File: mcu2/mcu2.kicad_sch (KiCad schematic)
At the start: 35 parts, among them J1 KF128-5.08, J2 Conn_01x30, J8 Conn_01x30, Q1 WSF3085, Q2 PL4009, Q3 PL4009, U1 Pico, U2 motor_driver, U3 max31865_module, U4 dcdc_module

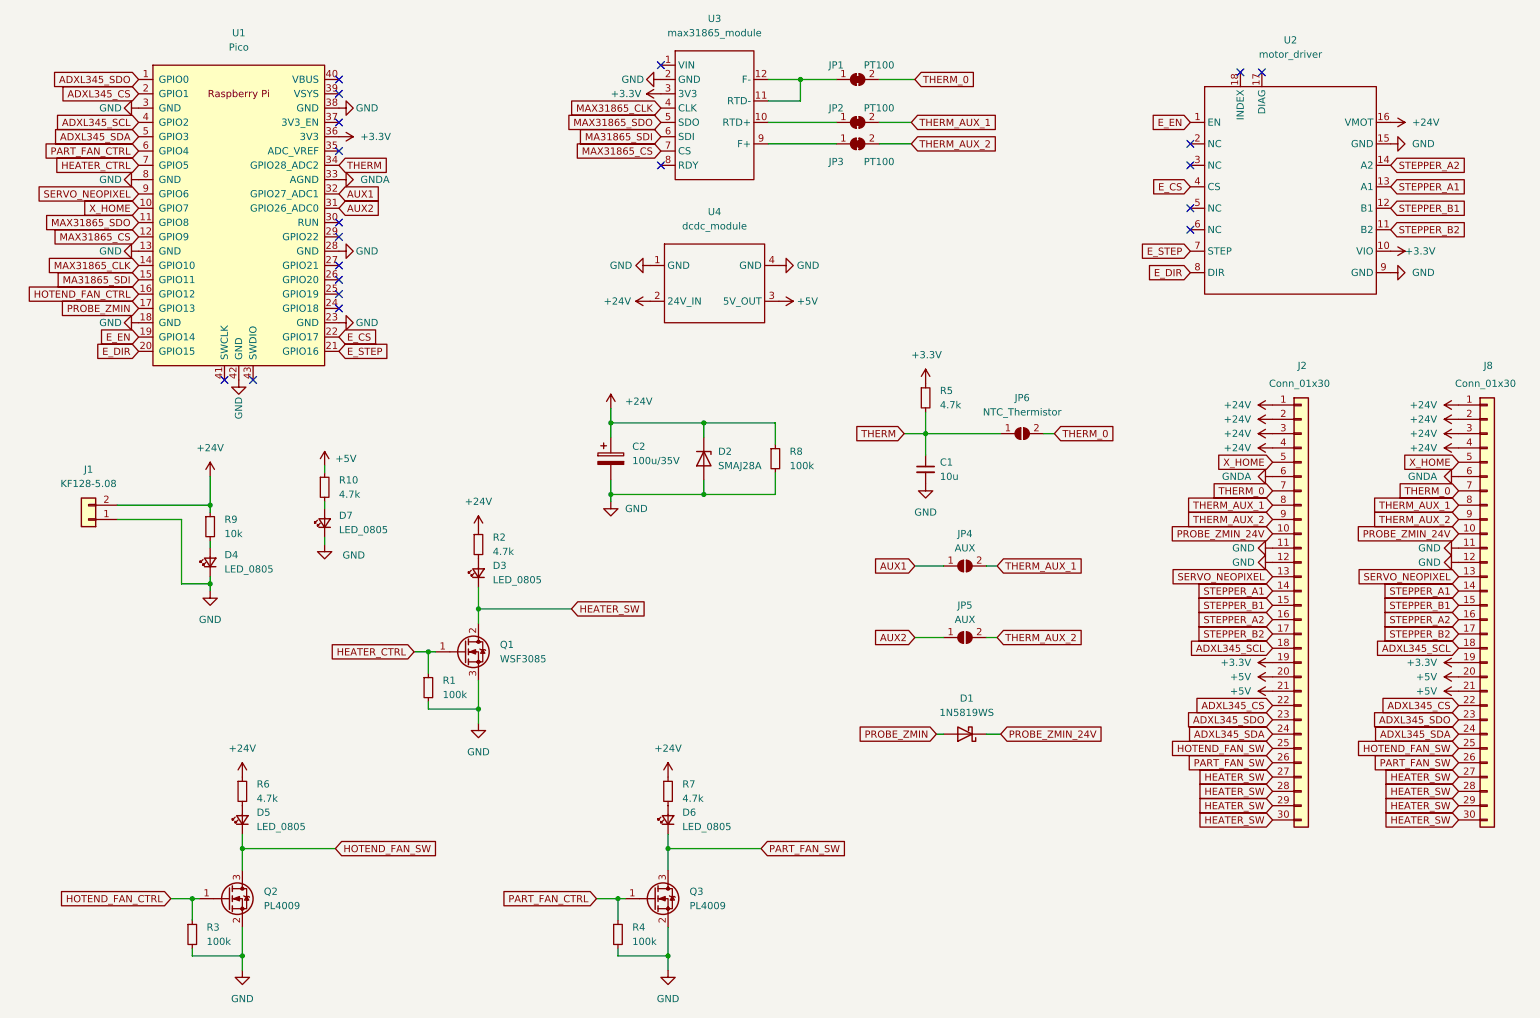
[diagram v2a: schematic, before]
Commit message: mcu2 wiring
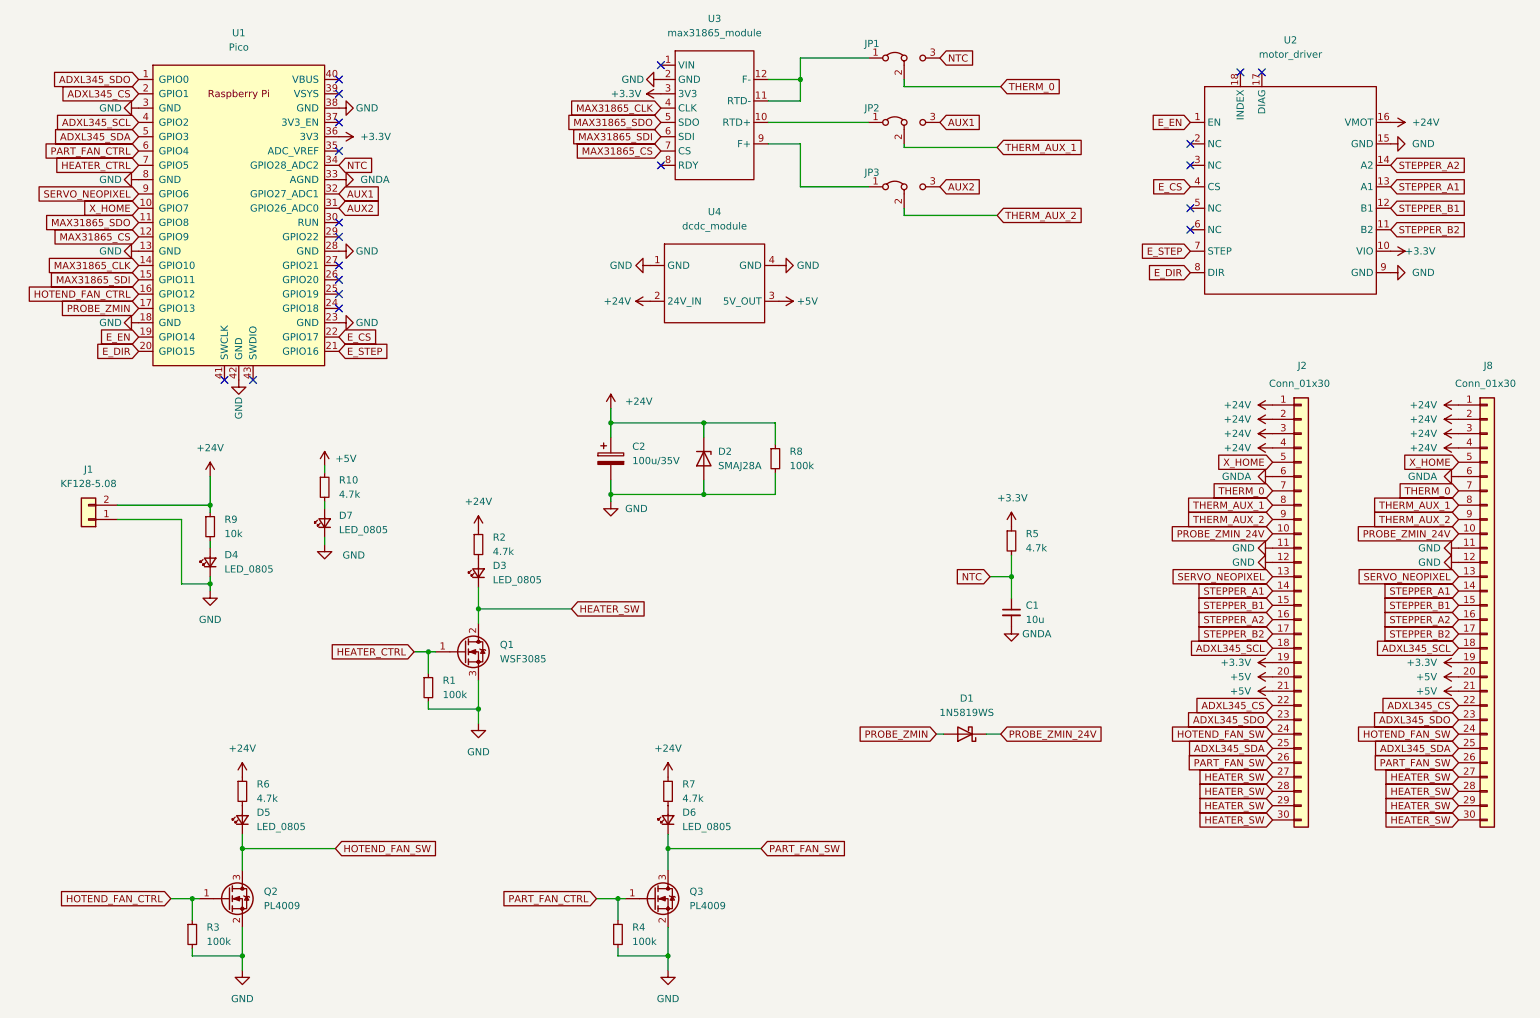
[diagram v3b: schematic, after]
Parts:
- removed JP1, JP2, JP3: PT100, Jumper:SolderJumper-2_P1.3mm_Bridged_RoundedPad1.0x1.5mm, symbol Jumper:SolderJumper_2_Bridged
- removed JP4, JP5: AUX, Jumper:SolderJumper-2_P1.3mm_Open_RoundedPad1.0x1.5mm, symbol Jumper:SolderJumper_2_Open
- removed JP6: NTC_Thermistor, Jumper:SolderJumper-2_P1.3mm_Open_RoundedPad1.0x1.5mm, symbol Jumper:SolderJumper_2_Open
- added JP1, JP2, JP3: Jumper_3_Bridged12, Jumper:SolderJumper-3_P1.3mm_Bridged12_RoundedPad1.0x1.5mm, symbol Jumper:Jumper_3_Bridged12
- J1: footprint FFCconnector:KF128-5.08 -> ffc_connectors:KF128-5.08
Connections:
- net ADXL345_SDA: now also J2.25 (Pin_25), J8.25 (Pin_25); no longer J2.24 (Pin_24), J8.24 (Pin_24)
- net AUX1: now also JP2.3 (B)
- net AUX2: now also JP3.3 (B)
- net GND: no longer C1.2
- net GNDA: now also C1.2
- net HOTEND_FAN_SW: now also J2.24 (Pin_24), J8.24 (Pin_24); no longer J2.25 (Pin_25), J8.25 (Pin_25)
- net THERM_0: now also JP1.2 (C)
- net THERM_AUX_1: now also JP2.2 (C)
- net THERM_AUX_2: now also JP3.2 (C)
- net at U3.10 (RTD+): now also JP2.1 (A)
- net at U3.11 (RTD-), U3.12 (F-): now also JP1.1 (A)
- net at U3.9 (F+): now also JP3.1 (A)
- net MA31865_SDI renamed MAX31865_SDI
- net THERM renamed NTC
- net NTC: now also JP1.3 (B)
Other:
- moved on the sheet: C1, R5
